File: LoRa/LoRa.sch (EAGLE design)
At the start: 35 parts, among them J1 UP2-AH-1-TH, U1 STM32L053C8T6, U2 RFM69HCW, U5 LM3671MF-3.3/NOPB, X1 uFL/SMA, Y1 ECS-80-S-4X

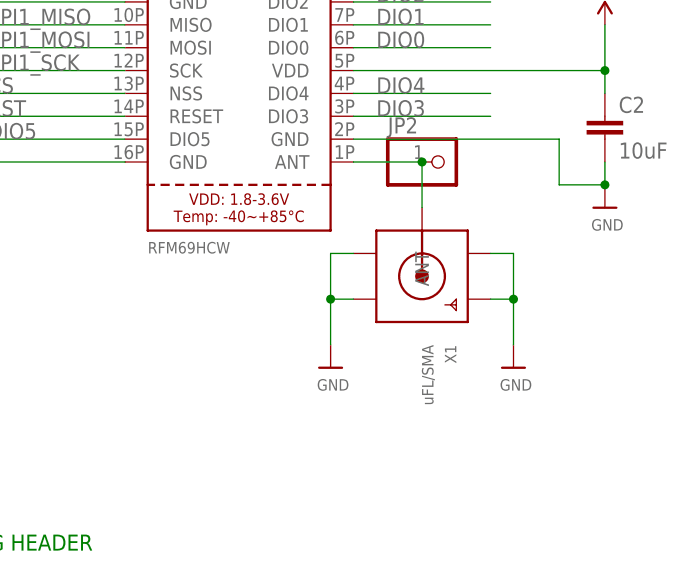
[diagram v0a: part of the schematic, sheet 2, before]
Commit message: Final touches
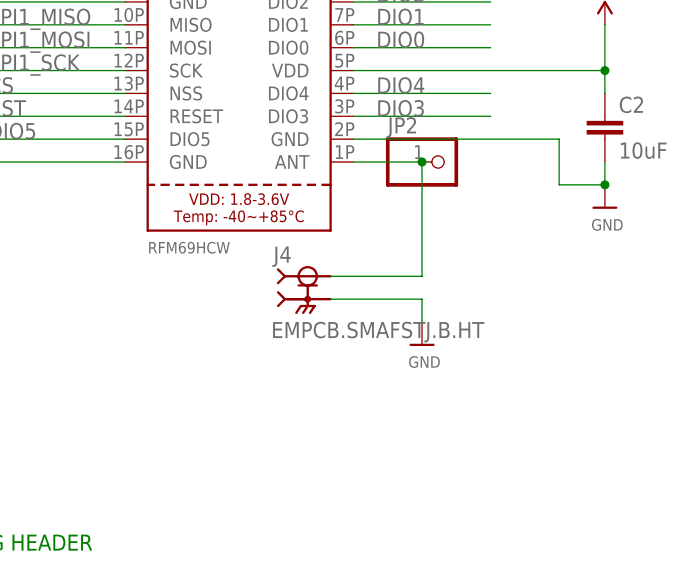
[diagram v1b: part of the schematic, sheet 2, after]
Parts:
- removed X1: uFL/SMA, microbuilder:SMACONNECTOR_EDGE_UFL
- added J4: EMPCB.SMAFSTJ.B.HT, EMPCB.SMAFSTJ.B.HT:EMPCB.SMAFSTJ.B.HT
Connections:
- net GND: now also J4.2; no longer X1.GND1, X1.GND2, X1.GND3, X1.GND4
- net N$1: now also J4.1; no longer X1.ANT
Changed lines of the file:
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@@
 <part name="U2" library="microbuilder" deviceset="RFM69HCW" device="_SMT" value="RFM69HCW"/>
 <part name="U$6" library="microbuilder" deviceset="GND" device=""/>
-<part name="X1" library="microbuilder" deviceset="SMACONNECTOR" device="_EDGE_UFL" value="uFL/SMA"/>
-<part name="U$7" library="microbuilder" deviceset="GND" device=""/>
-<part name="U$9" library="microbuilder" deviceset="GND" device=""/>
 <part name="JP2" library="microbuilder" deviceset="HEADER-1X1" device="ROUND"/>
 <part name="C2" library="SparkFun-Capacitors" library_urn="urn:adsk.eagle:library:510" deviceset="10UF" device="-0603-6.3V-20%" package3d_urn="urn:adsk.eagle:package:37414/1" value="10uF"/>
@@
 <part name="GND1" library="supply2" library_urn="urn:adsk.eagle:library:372" deviceset="GND" device=""/>
 <part name="R2" library="SparkFun-Resistors" library_urn="urn:adsk.eagle:library:532" deviceset="1KOHM" device="-0603-1/10W-1%" package3d_urn="urn:adsk.eagle:package:39650/1" value="1k"/>
+<part name="J4" library="EMPCB.SMAFSTJ.B.HT" deviceset="EMPCB.SMAFSTJ.B.HT" device=""/>
+<part name="U$17" library="microbuilder" deviceset="GND" device=""/>
 </parts>
 <sheets>
@@
 <instance part="U2" gate="G$1" x="210.82" y="210.82"/>
 <instance part="U$6" gate="G$1" x="251.46" y="195.58"/>
-<instance part="X1" gate="G$1" x="231.14" y="187.96" rot="R270"/>
-<instance part="U$7" gate="G$1" x="241.3" y="177.8"/>
-<instance part="U$9" gate="G$1" x="220.98" y="177.8"/>
 <instance part="JP2" gate="G$1" x="233.68" y="200.66"/>
 <instance part="C2" gate="G$1" x="251.46" y="203.2"/>
@@
 <attribute name="VALUE" x="131.064" y="172.72" size="1.778" layer="96" font="vector" rot="R90" align="top-center"/>
 </instance>
+<instance part="J4" gate="G$1" x="218.44" y="185.42"/>
+<instance part="U$17" gate="G$1" x="231.14" y="180.34"/>
 </instances>
 <busses>
@@
 <wire x1="251.46" y1="198.12" x2="251.46" y2="200.66" width="0.1524" layer="91"/>
 <junction x="251.46" y="198.12"/>
-</segment>
-<segment>
-<pinref part="X1" gate="G$1" pin="GND2"/>
-<pinref part="U$7" gate="G$1" pin="GND"/>
-<wire x1="238.76" y1="185.42" x2="241.3" y2="185.42" width="0.1524" layer="91"/>
-<wire x1="241.3" y1="185.42" x2="241.3" y2="180.34" width="0.1524" layer="91"/>
-<pinref part="X1" gate="G$1" pin="GND1"/>
-<wire x1="238.76" y1="190.5" x2="241.3" y2="190.5" width="0.1524" layer="91"/>
-<wire x1="241.3" y1="190.5" x2="241.3" y2="185.42" width="0.1524" layer="91"/>
-<junction x="241.3" y="185.42"/>
-</segment>
-<segment>
-<pinref part="X1" gate="G$1" pin="GND4"/>
-<pinref part="U$9" gate="G$1" pin="GND"/>
-<wire x1="223.52" y1="185.42" x2="220.98" y2="185.42" width="0.1524" layer="91"/>
-<wire x1="220.98" y1="185.42" x2="220.98" y2="180.34" width="0.1524" layer="91"/>
-<pinref part="X1" gate="G$1" pin="GND3"/>
-<wire x1="223.52" y1="190.5" x2="220.98" y2="190.5" width="0.1524" layer="91"/>
-<wire x1="220.98" y1="190.5" x2="220.98" y2="185.42" width="0.1524" layer="91"/>
-<junction x="220.98" y="185.42"/>
 </segment>
 <segment>
@@
 <pinref part="GND1" gate="GND" pin="GND"/>
 <wire x1="129.54" y1="154.94" x2="129.54" y2="152.4" width="0.1524" layer="91"/>
+</segment>
+<segment>
+<pinref part="J4" gate="G$1" pin="2"/>
+<wire x1="220.98" y1="185.42" x2="231.14" y2="185.42" width="0.1524" layer="91"/>
+<pinref part="U$17" gate="G$1" pin="GND"/>
+<wire x1="231.14" y1="182.88" x2="231.14" y2="185.42" width="0.1524" layer="91"/>
 </segment>
 </net>
@@
 <net name="N$1" class="0">
 <segment>
-<pinref part="X1" gate="G$1" pin="ANT"/>
 <wire x1="223.52" y1="200.66" x2="231.14" y2="200.66" width="0.1524" layer="91"/>
-<wire x1="231.14" y1="200.66" x2="231.14" y2="195.58" width="0.1524" layer="91"/>
 <pinref part="U2" gate="G$1" pin="ANT"/>
 <pinref part="JP2" gate="G$1" pin="1"/>
+<pinref part="J4" gate="G$1" pin="1"/>
+<wire x1="220.98" y1="187.96" x2="231.14" y2="187.96" width="0.1524" layer="91"/>
+<wire x1="231.14" y1="200.66" x2="231.14" y2="187.96" width="0.1524" layer="91"/>
 <junction x="231.14" y="200.66"/>
 </segment>
